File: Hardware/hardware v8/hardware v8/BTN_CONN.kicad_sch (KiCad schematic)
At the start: 15 parts, among them J3 OLED, J4 USB_C_Receptacle_USB2.0_14P

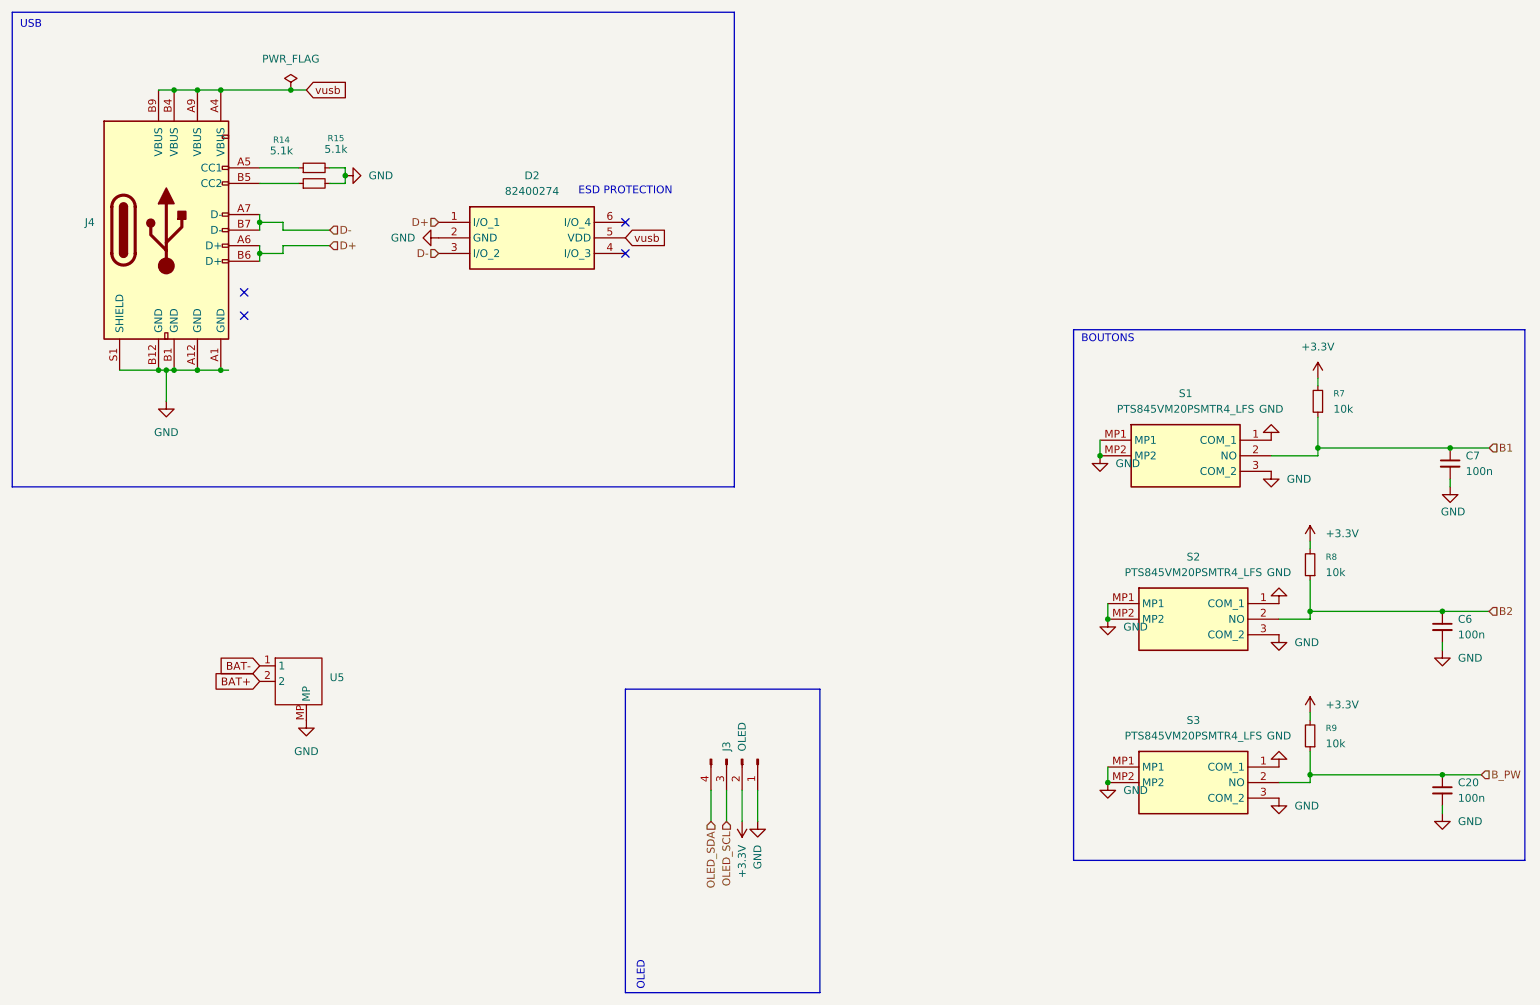
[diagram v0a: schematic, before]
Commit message: v8
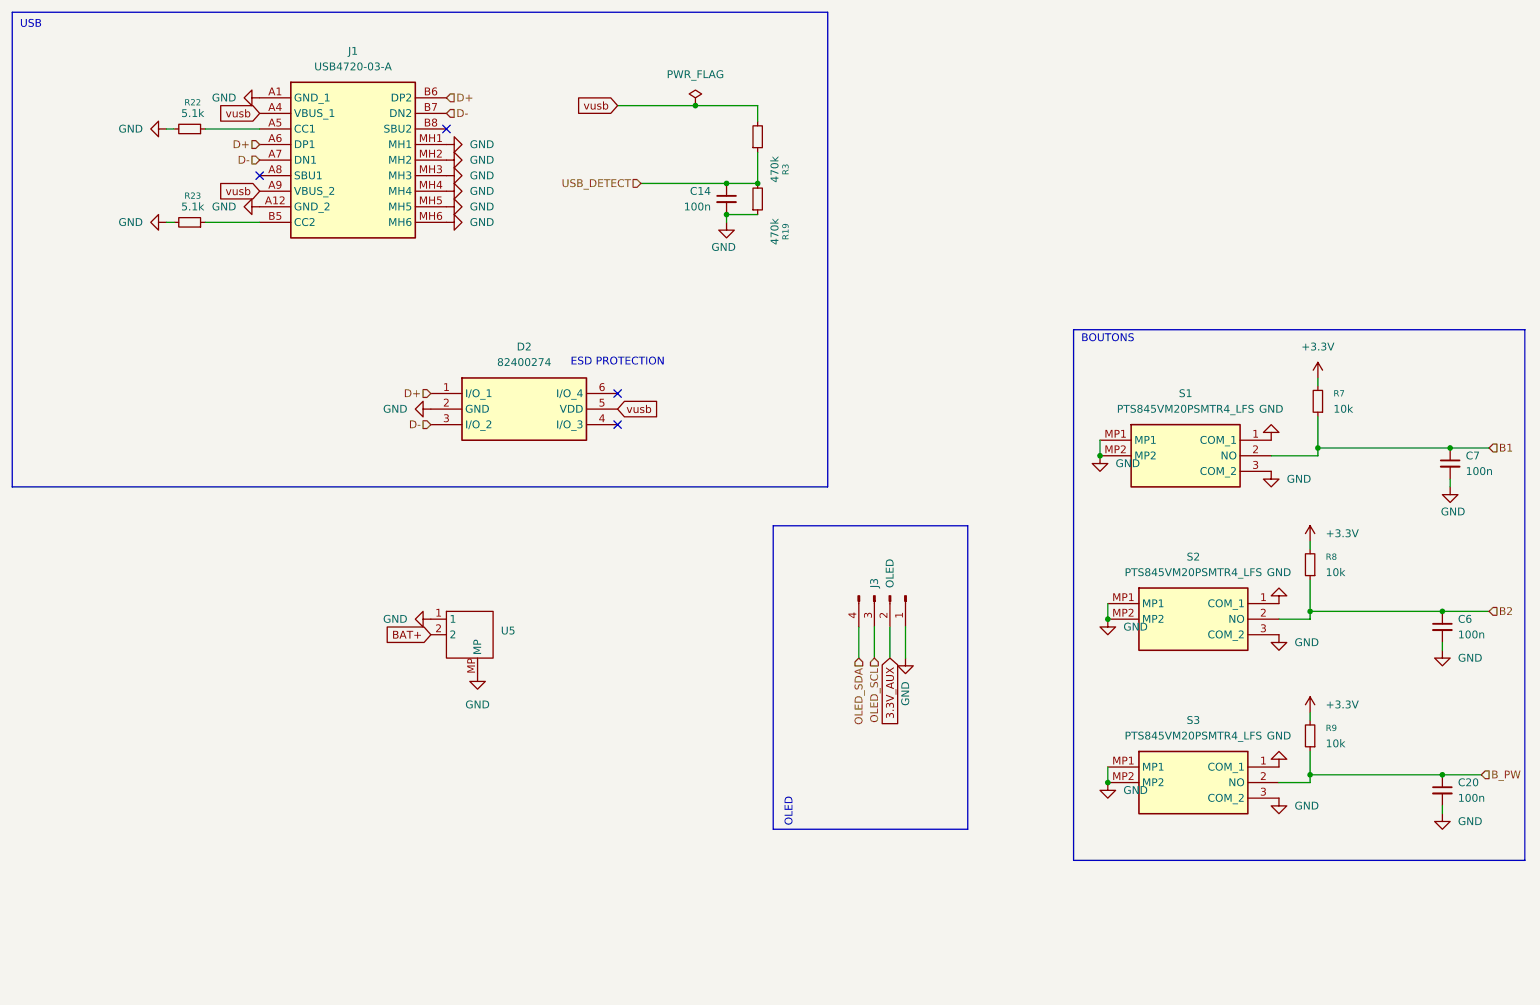
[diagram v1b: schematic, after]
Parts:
- removed J4: USB_C_Receptacle_USB2.0_14P, samacsys:USB4110GFA, symbol Vraielogousbcwurth:USB_C_Receptacle_USB2.0_14P
- removed R14, R15: 5.1k, Resistor_SMD:R_0201_0603Metric_Pad0.64x0.40mm_HandSolder, symbol Device:R_Small
- added C14: 100n, Capacitor_SMD:C_0201_0603Metric_Pad0.64x0.40mm_HandSolder, symbol Device:C_Small
- added J1: USB4720-03-A, samacsys2:USB472003A, symbol samacsys2:USB4720-03-A
- added R19, R3: 470k, Resistor_SMD:R_0201_0603Metric_Pad0.64x0.40mm_HandSolder, symbol Device:R_Small
- added R22, R23: 5.1k, Resistor_SMD:R_0201_0603Metric_Pad0.64x0.40mm_HandSolder, symbol Device:R_Small
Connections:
- net BAT- is gone; now on net GND: U5.1
- net +3.3V: no longer J3.2 (Pin_2)
- net D+: now also J1.A6 (DP1), J1.B6 (DP2)
- net D-: now also J1.A7 (DN1), J1.B7 (DN2)
- net GND: now also C14.2, J1.A1 (GND_1), J1.A12 (GND_2), J1.MH1, J1.MH2, J1.MH3, J1.MH4, J1.MH5, J1.MH6, R19.1, R22.2, R23.2
- net vusb: now also J1.A4 (VBUS_1), J1.A9 (VBUS_2), R3.2
- new net: J1.A5 (CC1), R22.1
- new net: J1.B5 (CC2), R23.1
- new net 3.3V_AUX: J3.2 (Pin_2)
- new net USB_DETECT: C14.1, R19.2, R3.1
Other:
- moved on the sheet: D2, J3, U5
